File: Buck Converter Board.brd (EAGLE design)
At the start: 120.6 x 47.7 mm, 8 parts, among them J1 POWERPOLE_POWER25A_HORIZONTAL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, J2 POWERPOLE_POWER25A_HORIZONTAL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, J3 POWERPOLE_POWER25A_HORIZONTAL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

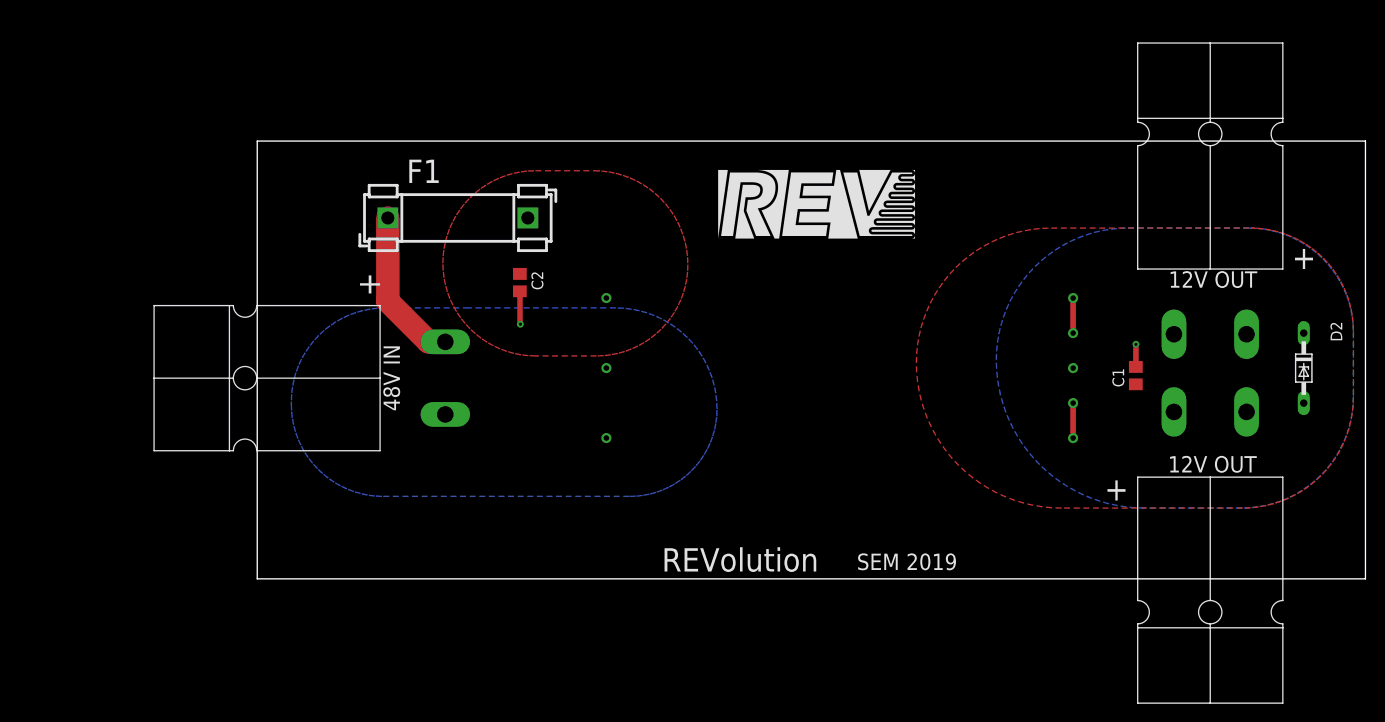
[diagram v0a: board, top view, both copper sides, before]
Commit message: changed buck board
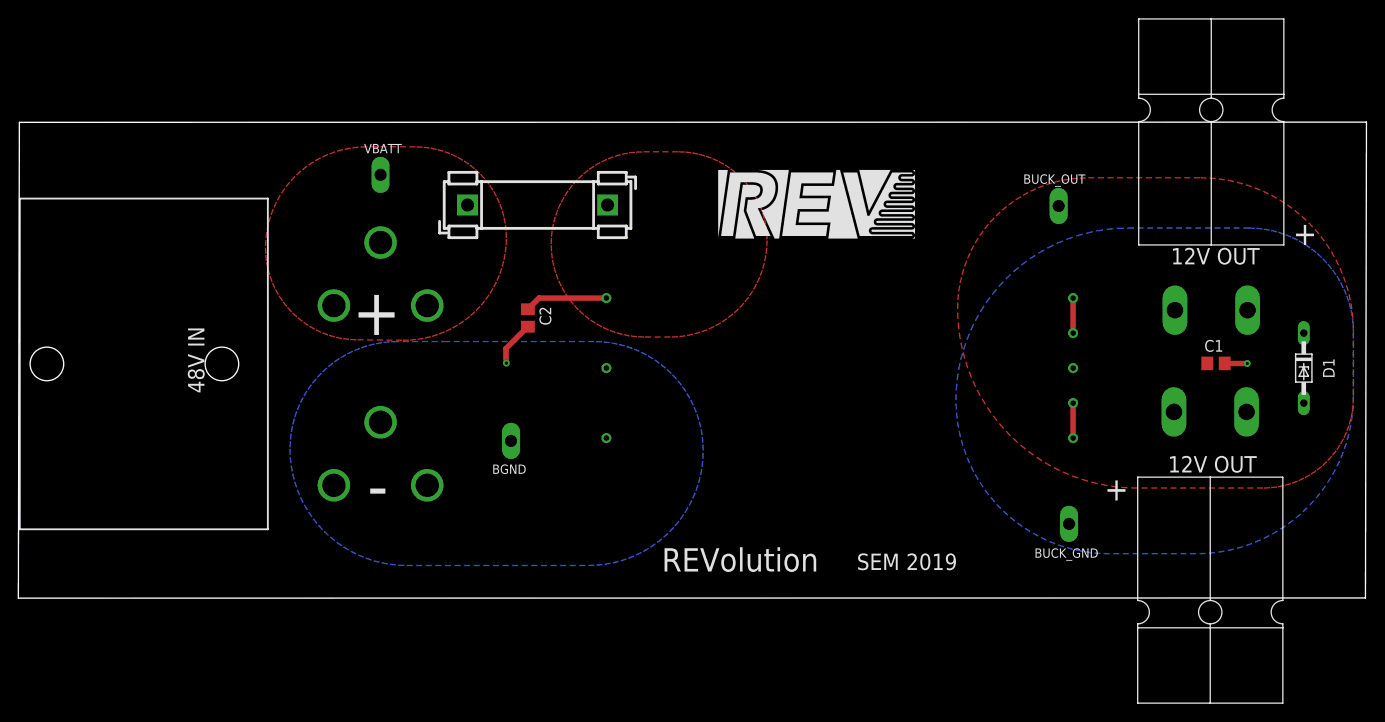
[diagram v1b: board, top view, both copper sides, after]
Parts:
- removed J1: POWERPOLE_POWER25A_HORIZONTAL_G2, powerpoles:POWERPOLE_PAIR_25A_HORIZ_G2
- added BGND, VBATT: VBATT, master_library:P1-13Y
- added BUCK_GND, BUCK_OUT: TEST_POINTSPAD1-13Y, master_library:P1-13Y
- added U$1: BATTERY, master_library:SB50POWER_CLAW
- D1: value (none) -> 15V
- moved C1 8.82 mm to (104.7, 23.4), turned to 0 degrees
- moved F1 8.79 mm to (23.3, 40.6)
- moved C2 3.95 mm to (29.8, 28.3)
- moved J2 2.62 mm to (104.2, 36.2)
- renumbered D2 to D1
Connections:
- net BGND: now also BGND.TP, U$1.NEG1, U$1.NEG2, U$1.NEG3; no longer J1.BLACK
- net OGND: now also BUCK_GND.TP
- net VBATT: now also U$1.POS1, U$1.POS2, U$1.POS3, VBATT.TP; no longer J1.RED
- net V_OUT: now also BUCK_OUT.TP
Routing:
- net VBATT: track 17.1 -> 0.00 mm
- net V_BATT_FUSED: track 0.00 -> 9.05 mm
- net BGND: track 3.60 -> 4.97 mm
- added copper zone on layer 1, net VBATT
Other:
- board size 120.6 x 47.7 mm -> 146.7 x 51.8 mm
